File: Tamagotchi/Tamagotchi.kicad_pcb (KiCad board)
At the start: 2 copper layers, 70.1 x 85.3 mm, 18 parts, among them SW1 SW_Push, SW2 SW_Push, SW3 SW_Push, SW4 SW_Push, SW5 SW_SPDT, U1 ESP32-C3-SuperMini, U2 SSD1306

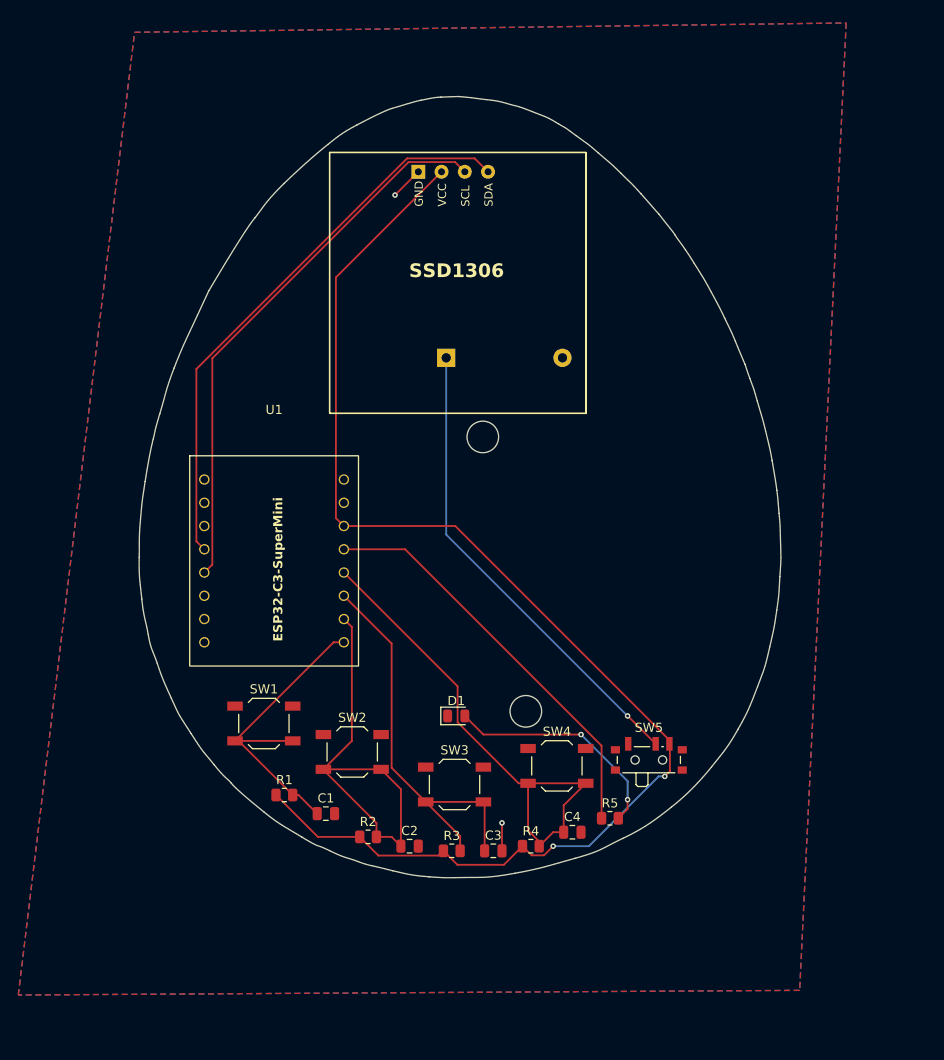
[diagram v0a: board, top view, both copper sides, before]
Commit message: updated Tamagotchi
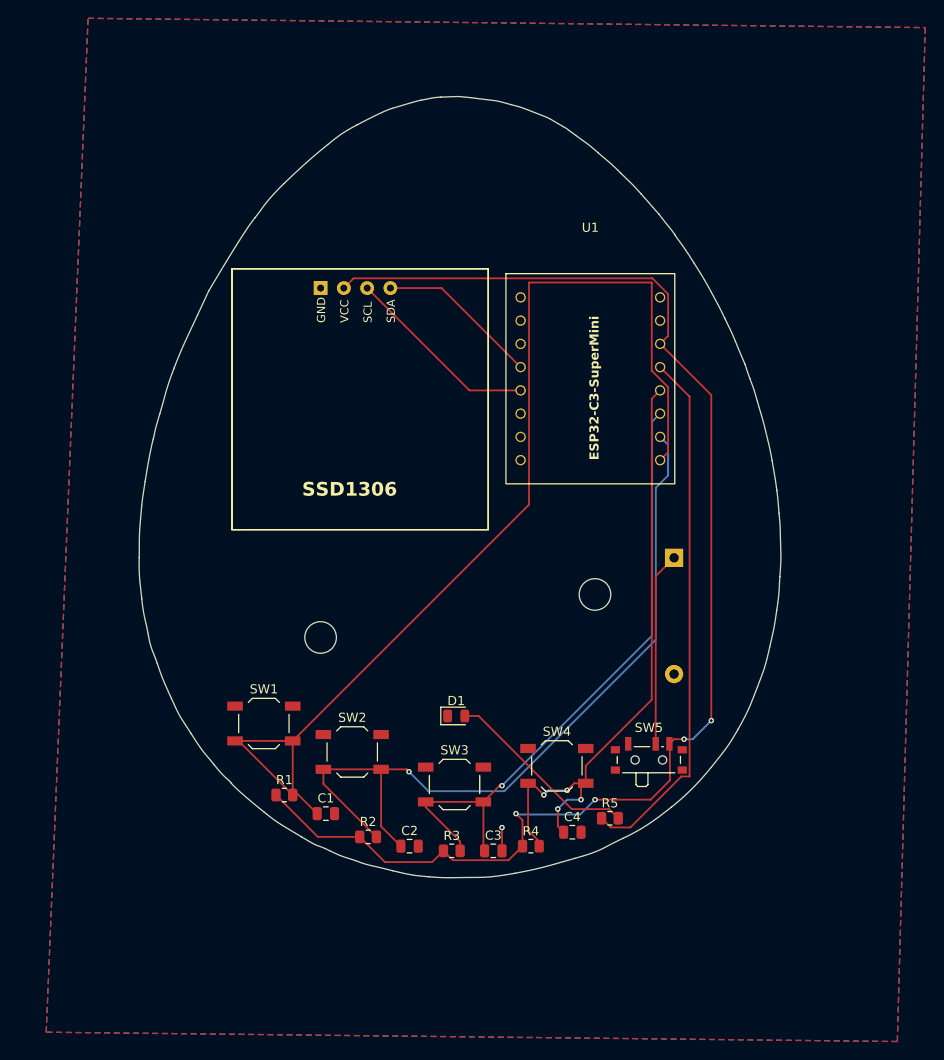
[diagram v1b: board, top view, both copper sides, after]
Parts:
- moved U1 39.9 mm to (160.0, 91.7)
- moved BT1 33.1 mm to (169.2, 111.3), turned to 180 degrees
- moved U2 16.6 mm to (134.4, 90.7)
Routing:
- net Net-(U1-GPIO0): track 34.9 -> 118.7 mm
- net Net-(U1-GPIO8): track 62.0 -> 17.8 mm
- net Net-(U1-GPIO1): track 46.5 -> 86.3 mm, vias 0 -> 1
- net Net-(U1-GPIO9): track 60.7 -> 21.4 mm
- net Net-(BT1-+): track 51.7 -> 21.2 mm, vias 1 -> 0
- net Net-(U1-GPIO2): track 44.8 -> 69.2 mm, vias 0 -> 1
- net Net-(U1-GPIO3): track 55.3 -> 68.8 mm, vias 0 -> 4
- net Net-(U1-GPIO4): track 45.0 -> 58.4 mm
- net Net-(SW5-C): track 144.2 -> 149.2 mm, vias 2 -> 4
- net GND: track 6.64 -> 2.54 mm, vias 2 -> 1
- net Net-(D1-A): track 25.2 -> 21.4 mm, vias 2 -> 0
